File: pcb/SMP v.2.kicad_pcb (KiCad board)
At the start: 2 copper layers, 123.8 x 58.7 mm, 21 parts, among them U1 Elite-C

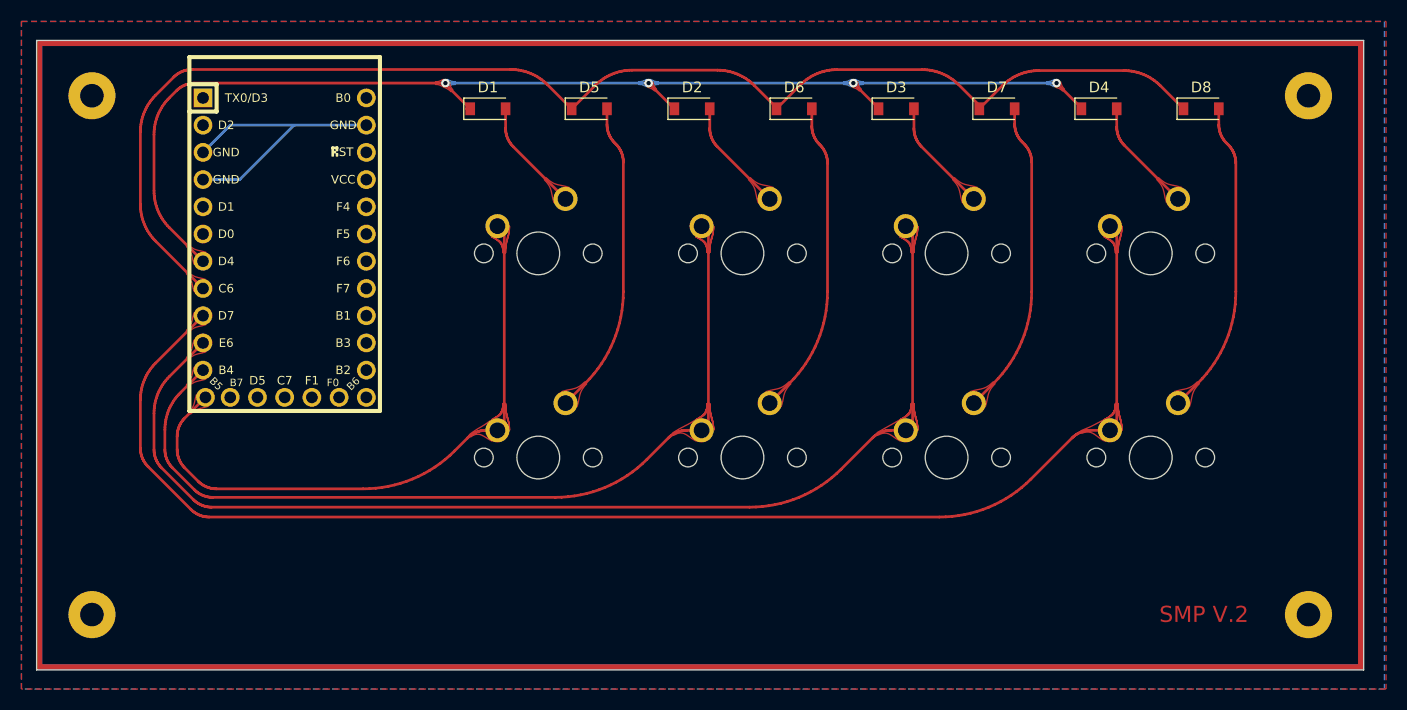
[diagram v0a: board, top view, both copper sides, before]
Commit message: WIP: on board mcu
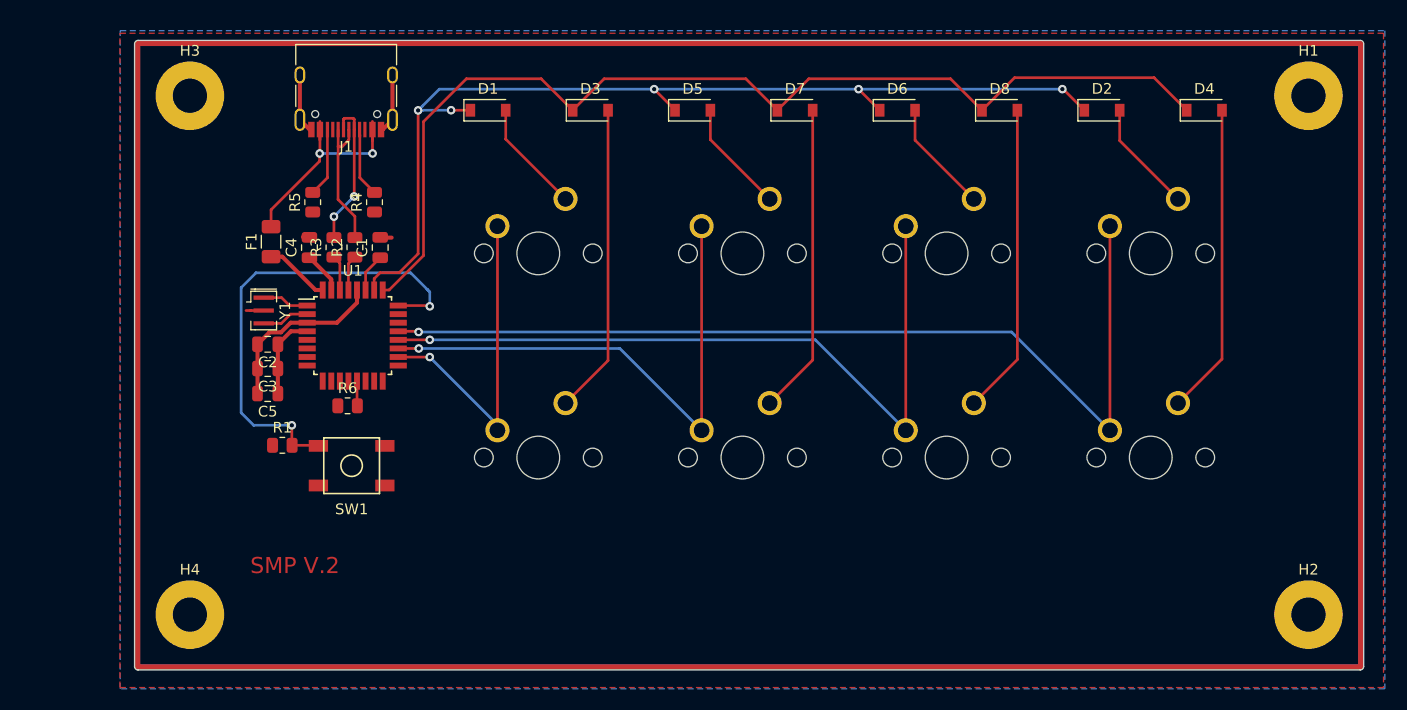
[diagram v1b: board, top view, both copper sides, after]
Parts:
- removed ? (x3), REF**: MountingHole_2.2mm_M2_Pad, MountingHole:MountingHole_2.2mm_M2_Pad
- added C1: 1uF, Capacitor_SMD:C_0805_2012Metric, F.Cu at (64.3, 44.5)
- added C2: 0.1uF, Capacitor_SMD:C_0805_2012Metric, F.Cu at (53.8, 53.6)
- added C3: 0.1uF, Capacitor_SMD:C_0805_2012Metric, F.Cu at (53.8, 55.8)
- added C4: 0.1uF, Capacitor_SMD:C_0805_2012Metric, F.Cu at (57.7, 44.5)
- added C5: 10uF, Capacitor_SMD:C_0805_2012Metric, F.Cu at (53.8, 58.2)
- added F1: 500mA, Fuse:Fuse_1206_3216Metric, F.Cu at (54.1, 44.0)
- added H1: MountingHole_Pad, MountingHole:MountingHole_3.2mm_M3_Pad, F.Cu at (150.9, 30.4)
- added H2: MountingHole_Pad, MountingHole:MountingHole_3.2mm_M3_Pad, F.Cu at (150.9, 78.8)
- added H3: MountingHole_Pad, MountingHole:MountingHole_3.2mm_M3_Pad, F.Cu at (46.5, 30.4)
- added H4: MountingHole_Pad, MountingHole:MountingHole_3.2mm_M3_Pad, F.Cu at (46.5, 78.8)
- added J1: USB_C_Receptacle_USB2.0, Connector_USB:USB_C_Receptacle_HRO_TYPE-C-31-M-12, F.Cu at (61.1, 29.5)
- added R1: 10k, Resistor_SMD:R_0805_2012Metric, F.Cu at (55.2, 63.0)
- added R2: 22, Resistor_SMD:R_0805_2012Metric, F.Cu at (61.9, 44.5)
- added R3: 22, Resistor_SMD:R_0805_2012Metric, F.Cu at (60.0, 44.5)
- added R4: 5.1k, Resistor_SMD:R_0805_2012Metric, F.Cu at (63.8, 40.3)
- added R5: 5.1k, Resistor_SMD:R_0805_2012Metric, F.Cu at (58.0, 40.3)
- added R6: 10k, Resistor_SMD:R_0805_2012Metric, F.Cu at (61.2, 59.3)
- added SW1: SW_Push, random-keyboard-parts:SKQG-1155865, F.Cu at (61.6, 64.9)
- added Y1: 16MHz, Crystal:Resonator_SMD_muRata_CSTxExxV-3Pin_3.0x1.1mm, F.Cu at (53.4, 50.4)
- U1: value Elite-C -> ATmega32U2-AU; footprint Keebio-Parts:Elite-C -> Package_QFP:TQFP-32_7x7mm_P0.8mm
- moved D2 38.3 mm to (131.6, 31.7)
- moved D3 28.5 mm to (83.9, 31.7)
- moved D7 18.8 mm to (103.0, 31.7)
- moved D8 18.8 mm to (122.1, 31.7)
- moved U1 10.4 mm to (61.7, 52.8), turned to 0 degrees
- moved D4 9.82 mm to (141.2, 31.7)
- moved D5 9.65 mm to (93.4, 31.7)
- moved D6 9.63 mm to (112.5, 31.7)
- moved D1 0.14 mm to (74.3, 31.7)
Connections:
- D1 pad 1: ROW0 -> ROW1
- D2 pad 1: ROW0 -> ROW1
- D7 pad 1: ROW1 -> ROW0
- D8 pad 1: ROW1 -> ROW0
- MX2 pad 2: Net-(D2-Pad2) -> Net-(D5-Pad2)
- MX3 pad 2: Net-(D3-Pad2) -> Net-(D6-Pad2)
- MX4 pad 2: Net-(D4-Pad2) -> Net-(D2-Pad2)
- MX5 pad 2: Net-(D5-Pad2) -> Net-(D3-Pad2)
- MX6 pad 2: Net-(D6-Pad2) -> Net-(D7-Pad2)
- MX7 pad 2: Net-(D7-Pad2) -> Net-(D8-Pad2)
- MX8 pad 2: Net-(D8-Pad2) -> Net-(D4-Pad2)
- U1 pad 10: COL2 -> Net-(U1-Pad10)
- U1 pad 11: COL1 -> Net-(U1-Pad11)
- U1 pad 12: COL0 -> Net-(U1-Pad12)
- U1 pad 18: Net-(U1-Pad18) -> COL0
- U1 pad 19: Net-(U1-Pad19) -> COL1
- U1 pad 20: Net-(U1-Pad20) -> COL2
- U1 pad 21: Net-(U1-Pad21) -> COL3
- U1 pad 23: GND -> Net-(U1-Pad23)
- U1 pad 25: Net-(U1-Pad25) -> ROW0
- U1 pad 26: Net-(U1-Pad26) -> ROW1
- U1 pad 28: Net-(U1-Pad28) -> GND
- U1 pad 4: GND -> +5V
- U1 pad 7: ROW0 -> Net-(U1-Pad7)
- U1 pad 8: ROW1 -> Net-(U1-Pad8)
- U1 pad 9: COL3 -> Net-(U1-Pad9)
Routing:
- net Net-(R1-Pad2): track 0.00 -> 44.8 mm, vias 0 -> 2
- net COL3: track 130.9 -> 89.3 mm, vias 0 -> 1
- net COL2: track 106.6 -> 69.9 mm, vias 0 -> 1
- net ROW1: track 126.9 -> 93.7 mm, vias 0 -> 5
- net COL1: track 82.8 -> 50.6 mm, vias 0 -> 1
- net COL0: track 58.9 -> 31.4 mm, vias 0 -> 1
- net Net-(F1-Pad2): track 0.00 -> 22.2 mm, vias 0 -> 2
- net Net-(D6-Pad2): track 30.5 -> 10.5 mm
- net Net-(D5-Pad2): track 29.6 -> 10.6 mm
- net Net-(D4-Pad2): track 10.7 -> 29.0 mm
- net Net-(D3-Pad2): track 10.6 -> 29.0 mm
- net +5V: track 0.00 -> 17.8 mm
- net ROW0: track 114.5 -> 99.1 mm, vias 4 -> 0
- net D-: track 0.00 -> 13.9 mm, vias 0 -> 2
- net D+: track 0.00 -> 13.2 mm
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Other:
- board size 123.8 x 58.7 mm -> 114.7 x 58.7 mm
